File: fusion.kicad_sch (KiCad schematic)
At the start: 49 parts, among them J1 Conn_01x04_Female, J2 USB_C_Receptacle_USB2.0, J3 Conn_01x12_MountingPin, J4 Conn_01x12_MountingPin, K19 diode-choc, K20 diode-choc, K21 diode-choc, K22 diode-choc, K23 diode-choc, K24 diode-choc, K25 diode-choc, K26 diode-choc, K27 diode-choc, K28 diode-choc, K29 diode-choc, K30 diode-choc, K31 diode-choc, K32 diode-choc, K33 diode-choc, K34 diode-choc, K35 diode-choc, K36 diode-choc, K37 diode-choc, K38 diode-choc, SW1 SW_Push, U1 Holyiot_18010, U2 MT25QL128ABA1ESE

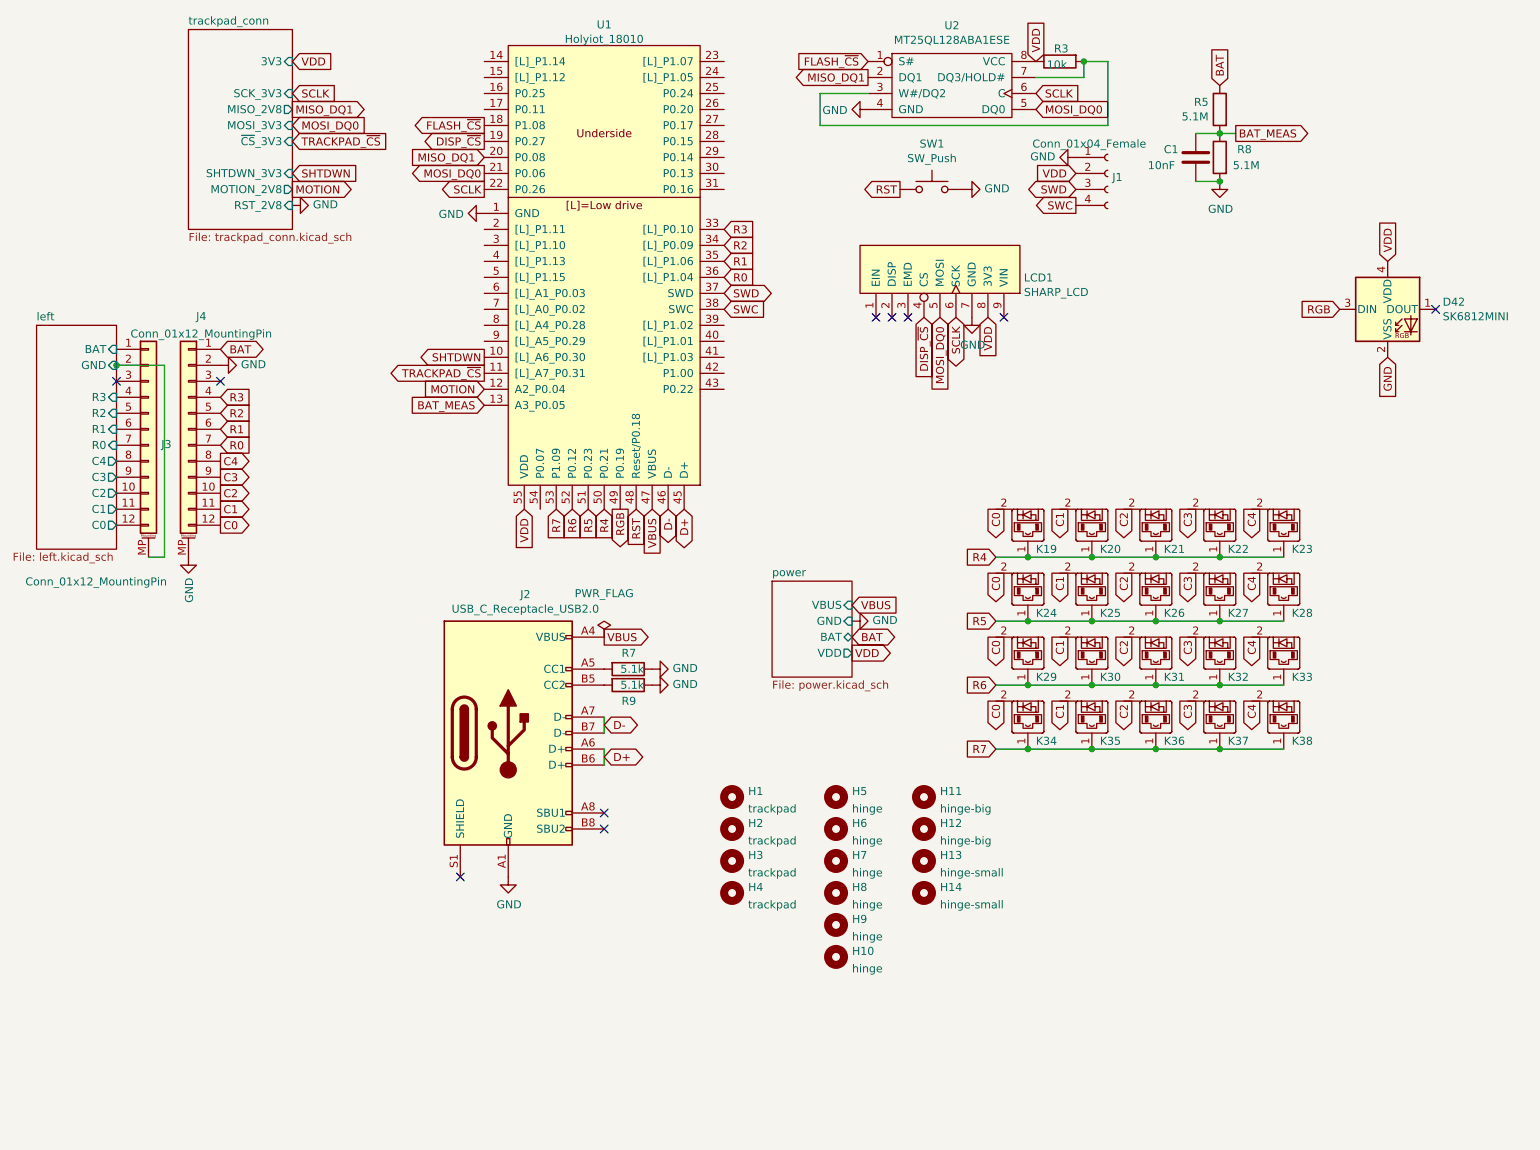
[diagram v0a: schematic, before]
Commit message: final?
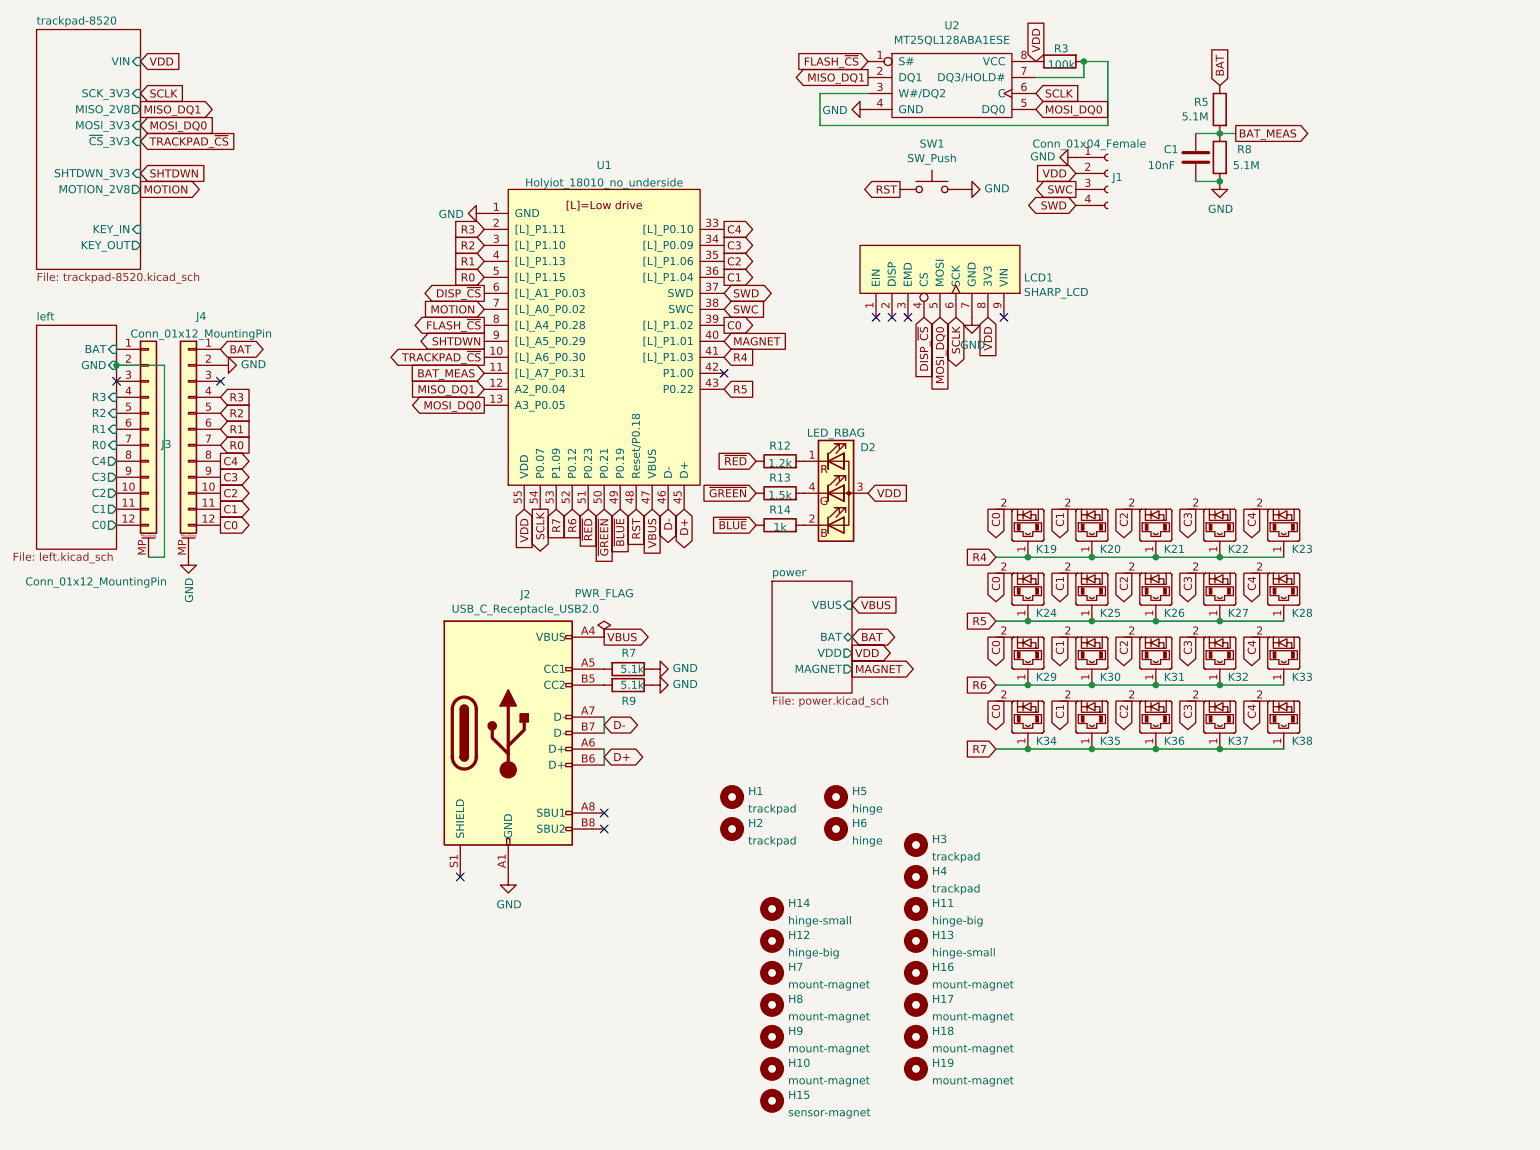
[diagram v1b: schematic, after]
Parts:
- removed D42: SK6812MINI, LED_SMD:LED_SK6812MINI_PLCC4_3.5x3.5mm_P1.75mm, symbol LED:SK6812MINI
- removed U1: Holyiot_18010, keeb-libs:Holyiot-18010, symbol keeb-libs:Holyiot_18010
- added D2: LED_RBAG, fusion:FM-B2020RGBA, symbol Device:LED_RBAG
- added H15: sensor-magnet, fusion:sensor-magnet, symbol Mechanical:MountingHole
- added H16, H17, H18, H19: mount-magnet, fusion:mount-magnet, symbol Mechanical:MountingHole
- added R12: 1.2k, Resistor_SMD:R_0603_1608Metric, symbol Device:R
- added R13: 1.5k, Resistor_SMD:R_0603_1608Metric, symbol Device:R
- added R14: 1k, Resistor_SMD:R_0603_1608Metric, symbol Device:R
- added U1: Holyiot_18010_no_underside, keeb-libs:Holyiot-18010-no-underside, symbol keeb-libs:Holyiot_18010_no_underside
- H10, H7, H8, H9: value hinge -> mount-magnet; footprint fusion:hinge -> fusion:mount-magnet
- J1: footprint keeb-libs:debug-port -> keeb-libs:debug-port-single-side
- R3: value 10k -> 100k
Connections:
- net BAT_MEAS: now also U1.11 ([L]_A7_P0.31)
- net C0: now also U1.39 ([L]_P1.02)
- net C1: now also U1.36 ([L]_P1.04)
- net C2: now also U1.35 ([L]_P1.06)
- net C3: now also U1.34 ([L]_P0.09)
- net C4: now also U1.33 ([L]_P0.10)
- net D+: now also U1.45 (D+)
- net D-: now also U1.46 (D-)
- net DISP_~{CS}: now also U1.6 ([L]_A1_P0.03)
- net FLASH_~{CS}: now also U1.8 ([L]_A4_P0.28)
- net GND: now also U1.1 (GND), U1.32 (GND), U1.44 (GND)
- net MISO_DQ1: now also U1.12 (A2_P0.04)
- net MOSI_DQ0: now also U1.13 (A3_P0.05)
- net MOTION: now also U1.7 ([L]_A0_P0.02)
- net R0: now also U1.5 ([L]_P1.15)
- net R1: now also U1.4 ([L]_P1.13)
- net R2: now also U1.3 ([L]_P1.10)
- net R3: now also U1.2 ([L]_P1.11)
- net R4: now also U1.41 ([L]_P1.03)
- net R5: now also U1.43 (P0.22)
- net R6: now also U1.52 (P0.12)
- net R7: now also U1.53 (P1.09)
- net RST: now also U1.48 (Reset/P0.18)
- net SCLK: now also U1.54 (P0.07)
- net SHTDWN: now also U1.9 ([L]_A5_P0.29)
- net SWC: now also J1.3 (Pin_3), U1.38 (SWC); no longer J1.4 (Pin_4)
- net SWD: now also J1.4 (Pin_4), U1.37 (SWD); no longer J1.3 (Pin_3)
- net TRACKPAD_~{CS}: now also U1.10 ([L]_A6_P0.30)
- net VBUS: now also U1.47 (VBUS)
- net VDD: now also D2.3 (A), U1.55 (VDD)
- new net: D2.4 (GK), R13.2
- new net: D2.1 (RK), R12.2
- new net: D2.2 (BK), R14.2
- new net MAGNET: U1.40 ([L]_P1.01)
- new net ~{BLUE}: R14.1, U1.49 (P0.19)
- new net ~{GREEN}: R13.1, U1.50 (P0.21)
- new net ~{RED}: R12.1, U1.51 (P0.23)
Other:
- removed sheet trackpad_conn
- added sheet trackpad-8520 (trackpad-8520.kicad_sch)
- sheet power ports: added MAGNET; removed GND
- moved on the sheet: H11, H12, H13, H14, H3, H4

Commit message: backup
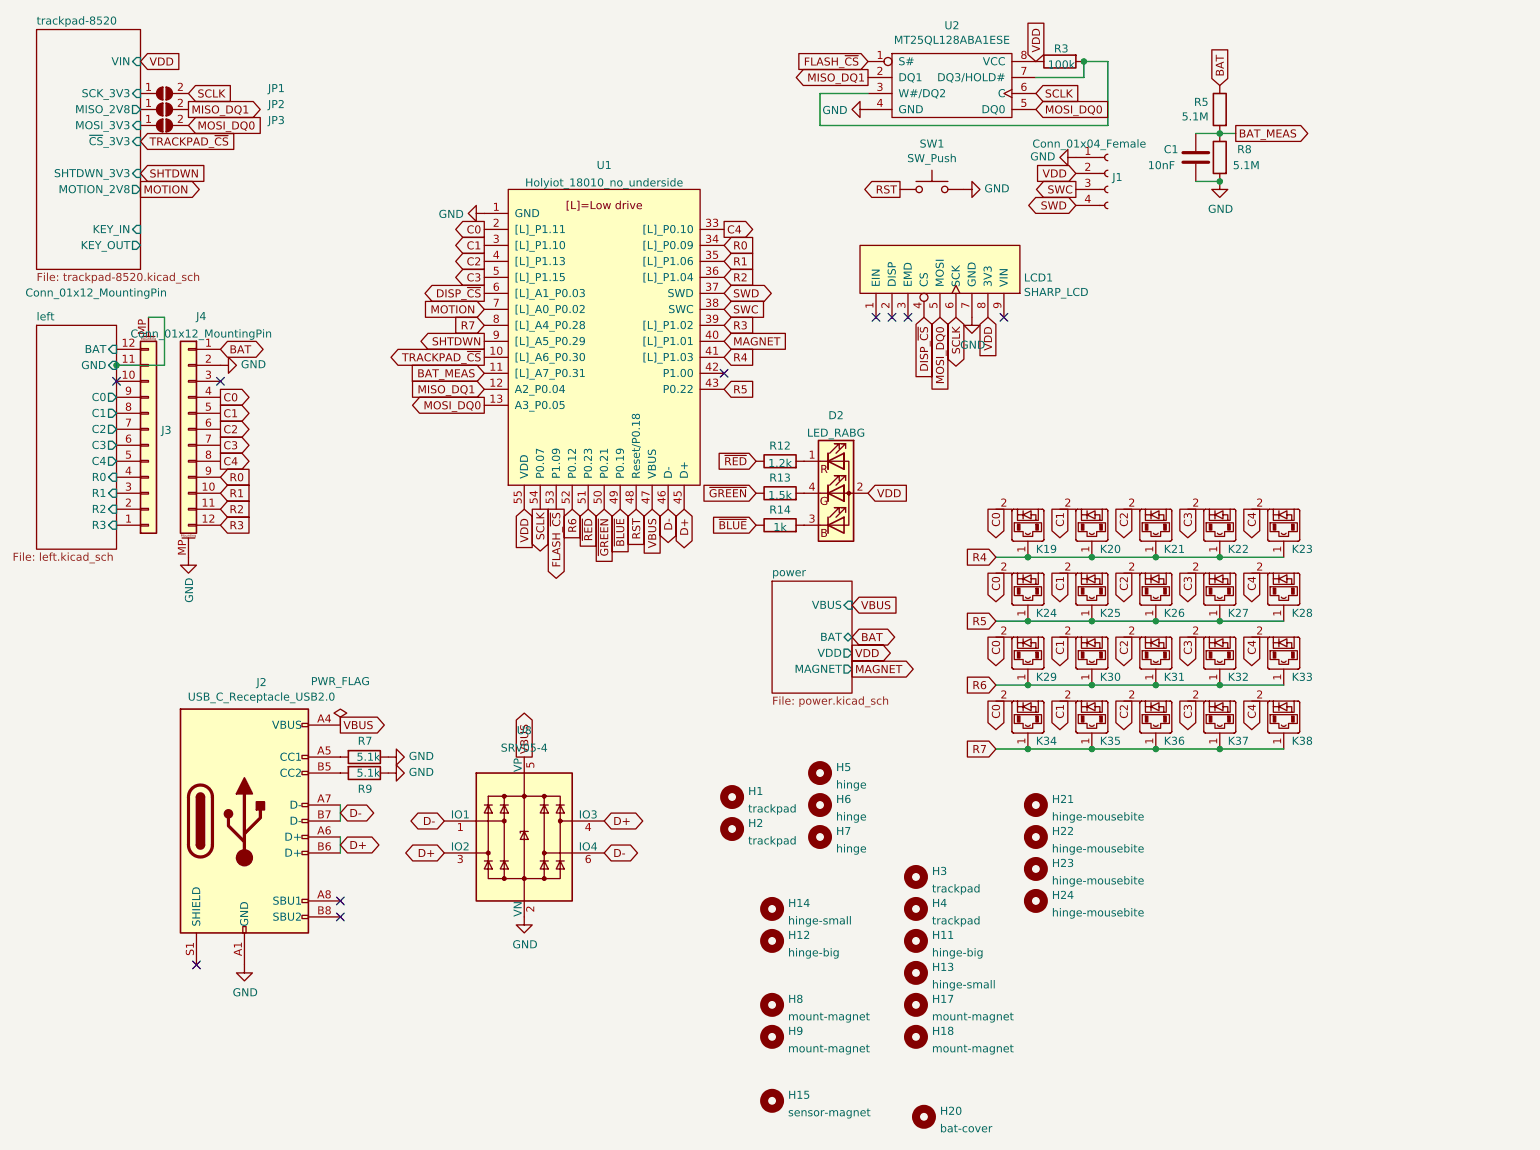
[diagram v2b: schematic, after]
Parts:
- removed D2: LED_RBAG, fusion:FM-B2020RGBA, symbol Device:LED_RBAG
- removed H10, H16, H19: mount-magnet, fusion:mount-magnet, symbol Mechanical:MountingHole
- added D2: LED_RABG, LED_SMD:LED_ASMB-KTF0-0A306, symbol Device:LED_RABG
- added H20: bat-cover, fusion:bat-cover, symbol Mechanical:MountingHole
- added H21, H22, H23, H24: hinge-mousebite, fusion:hinge-mousebite, symbol Mechanical:MountingHole
- added JP1, JP2, JP3: SolderJumper_2_Open, Jumper:SolderJumper-2_P1.3mm_Open_RoundedPad1.0x1.5mm, symbol Jumper:SolderJumper_2_Open
- added U8: SRV05-4, Package_TO_SOT_SMD:SOT-23-6, symbol Power_Protection:SRV05-4
- H7: value mount-magnet -> hinge; footprint fusion:mount-magnet -> fusion:hinge
- K19, K24, K29: footprint pg1232:pg1232-DSSL -> pg1232:pg1232-DSSN
- K20, K25, K30: footprint pg1232:pg1232-DSSR -> pg1232:pg1232-DSSL
- K22, K27, K32: footprint pg1232:pg1232-DSSL -> pg1232:pg1232-DSSR
- K23, K28, K33: footprint pg1232:pg1232-DSSN -> pg1232:pg1232-DSSL
- K34, K35: footprint pg1232:pg1232-DSS -> pg1232:pg1232-DSSN
- K37, K38: footprint pg1232:pg1232-DSSN -> pg1232:pg1232-DSS
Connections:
- net C0: now also J4.4 (Pin_4), U1.2 ([L]_P1.11); no longer J4.12 (Pin_12), U1.39 ([L]_P1.02)
- net C1: now also J4.5 (Pin_5), U1.3 ([L]_P1.10); no longer J4.11 (Pin_11), U1.36 ([L]_P1.04)
- net C2: now also J4.6 (Pin_6), U1.4 ([L]_P1.13); no longer J4.10 (Pin_10), U1.35 ([L]_P1.06)
- net C3: now also J4.7 (Pin_7), U1.5 ([L]_P1.15); no longer J4.9 (Pin_9), U1.34 ([L]_P0.09)
- net D+: now also U8.3 (IO2), U8.4 (IO3)
- net D-: now also U8.1 (IO1), U8.6 (IO4)
- net FLASH_~{CS}: now also U1.53 (P1.09); no longer U1.8 ([L]_A4_P0.28)
- net GND: now also U8.2 (VN)
- net MISO_DQ1: now also JP2.2 (B)
- net MOSI_DQ0: now also JP3.2 (B)
- net R0: now also J4.9 (Pin_9), U1.34 ([L]_P0.09); no longer J4.7 (Pin_7), U1.5 ([L]_P1.15)
- net R1: now also J4.10 (Pin_10), U1.35 ([L]_P1.06); no longer J4.6 (Pin_6), U1.4 ([L]_P1.13)
- net R2: now also J4.11 (Pin_11), U1.36 ([L]_P1.04); no longer J4.5 (Pin_5), U1.3 ([L]_P1.10)
- net R3: now also J4.12 (Pin_12), U1.39 ([L]_P1.02); no longer J4.4 (Pin_4), U1.2 ([L]_P1.11)
- net R7: now also U1.8 ([L]_A4_P0.28); no longer U1.53 (P1.09)
- net SCLK: now also JP1.2 (B)
- net VBUS: now also U8.5 (VP)
- net VDD: now also D2.2 (A)
- net left/BAT: now also J3.12 (Pin_12); no longer J3.1 (Pin_1)
- net left/C0: now also J3.9 (Pin_9); no longer J3.12 (Pin_12)
- net left/C1: now also J3.8 (Pin_8); no longer J3.11 (Pin_11)
- net left/C2: now also J3.7 (Pin_7); no longer J3.10 (Pin_10)
- net left/C3: now also J3.6 (Pin_6); no longer J3.9 (Pin_9)
- net left/C4: now also J3.5 (Pin_5); no longer J3.8 (Pin_8)
- net left/GND: now also J3.11 (Pin_11); no longer J3.2 (Pin_2)
- net left/R0: now also J3.4 (Pin_4); no longer J3.7 (Pin_7)
- net left/R1: now also J3.3 (Pin_3); no longer J3.6 (Pin_6)
- net left/R2: now also J3.2 (Pin_2); no longer J3.5 (Pin_5)
- net left/R3: now also J3.1 (Pin_1); no longer J3.4 (Pin_4)
- net at R13.2: now also D2.4 (GK)
- net at R12.2: now also D2.1 (RK)
- net at R14.2: now also D2.3 (BK)
- new net trackpad-8520/MISO_2V8: JP2.1 (A)
- new net trackpad-8520/MOSI_3V3: JP3.1 (A)
- new net trackpad-8520/SCK_3V3: JP1.1 (A)
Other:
- moved on the sheet: H11, H13, H3, H4, H5, H6, J2, J3, R7, R9
